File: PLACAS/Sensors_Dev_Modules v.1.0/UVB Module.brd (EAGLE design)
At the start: 25 x 25 mm, 5 parts

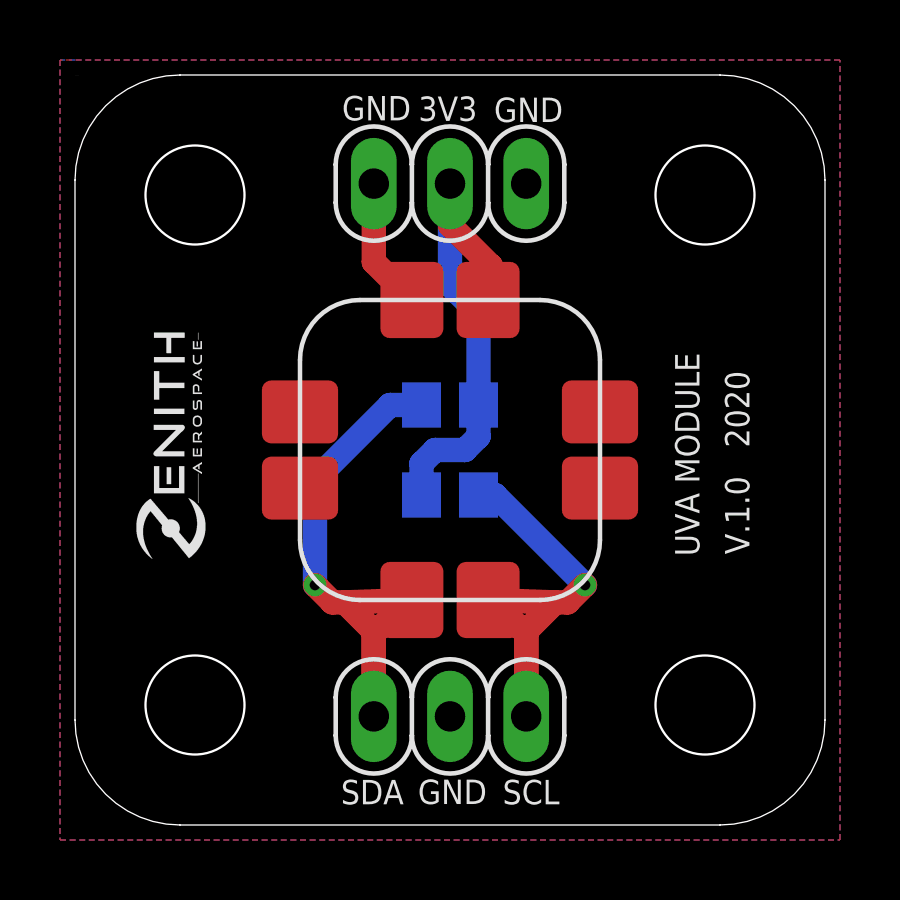
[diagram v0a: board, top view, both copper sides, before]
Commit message: Add files via upload
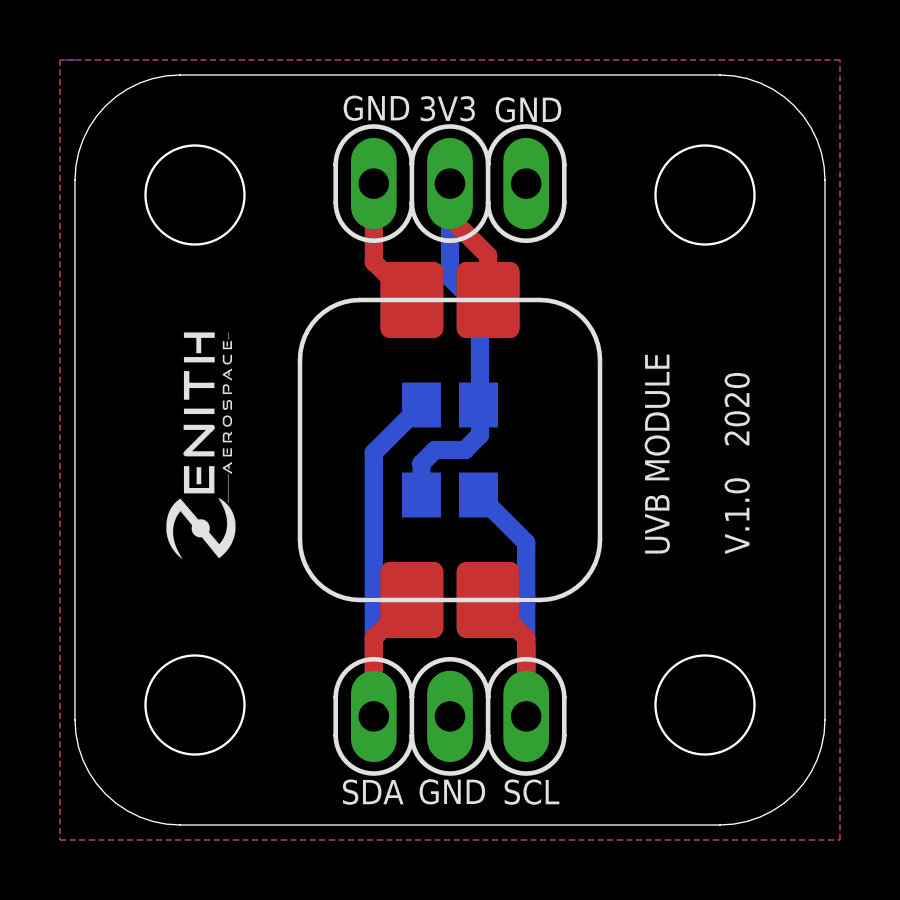
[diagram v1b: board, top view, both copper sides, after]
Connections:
- net GND: now also U$1.GND; no longer U$1.GND0, U$1.GND1, U$1.GND2, U$1.GND3, U$1.GND4
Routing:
- net N$4: track 20.2 -> 15.6 mm, vias 1 -> 0
- net N$5: track 16.9 -> 15.0 mm, vias 1 -> 0
- net +3V3: track 17.6 -> 16.7 mm
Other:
- board text added: "UVB MODULE"
- board text removed: "UVA MODULE"
